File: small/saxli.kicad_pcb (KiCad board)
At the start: 4 copper layers, 160.5 x 102.4 mm, 191 parts, among them IC1 PIC32MX350F256H-V_PT, IC2 SIM808, J1 78800-0001, J10 Conn_01x06_Female, J11 Conn_Coaxial, J12 Conn_Coaxial, J2 Screw_Terminal_01x02, J3 Micro_SD_Card, J4 Conn_01x05_Female, J5 Conn_02x04_Odd_Even, J6 RJ45_Amphenol_RJMG1BD3B8K1ANR, J7 Screw_Terminal_01x08, J8 Screw_Terminal_01x08, J9 Screw_Terminal_01x08, Q1 2N7002, Q2 2N7002, Q3 2N7002, U1 LM358, U10 TPS5430DDAR, U11 EL357N(C)(TA)-G, U12 EL357N(C)(TA)-G, U13 ASSR-1218, U14 ST485EBDR, U15 ASSR-1218, U16 SRV05-4, U18 ULN2003A, U2 LM7805_TO220, U20 TPS5430DDAR, U3 LD1117S33TR_SOT223, U4 ENC28J60x-SS, U5 AT25M02, U6 EL357N(C)(TA)-G, U7 EL357N(C)(TA)-G, U8 PCF8563T, U9 ISO1540, Y1 Crystal, Y2 Crystal

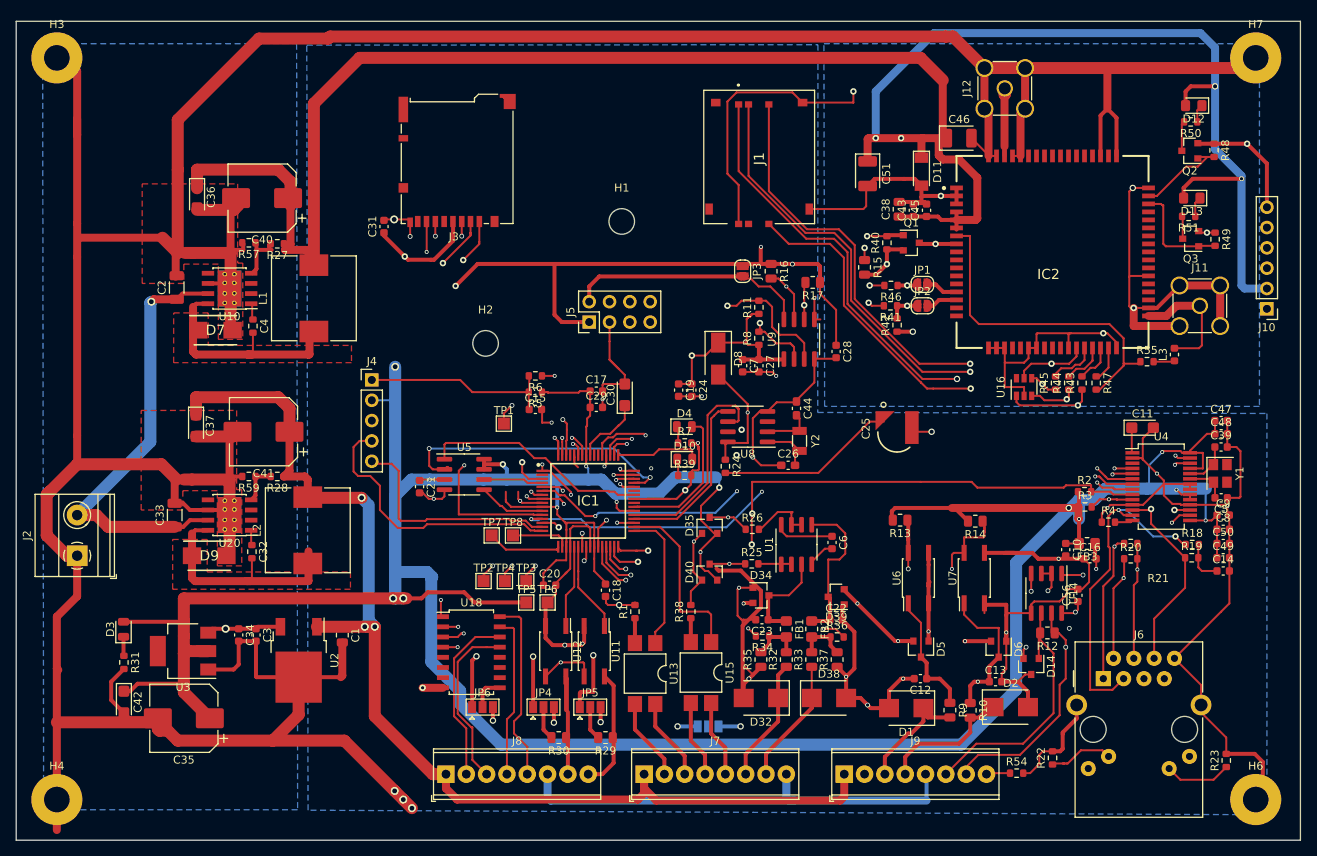
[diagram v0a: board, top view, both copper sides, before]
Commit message: ENC28j60 routed
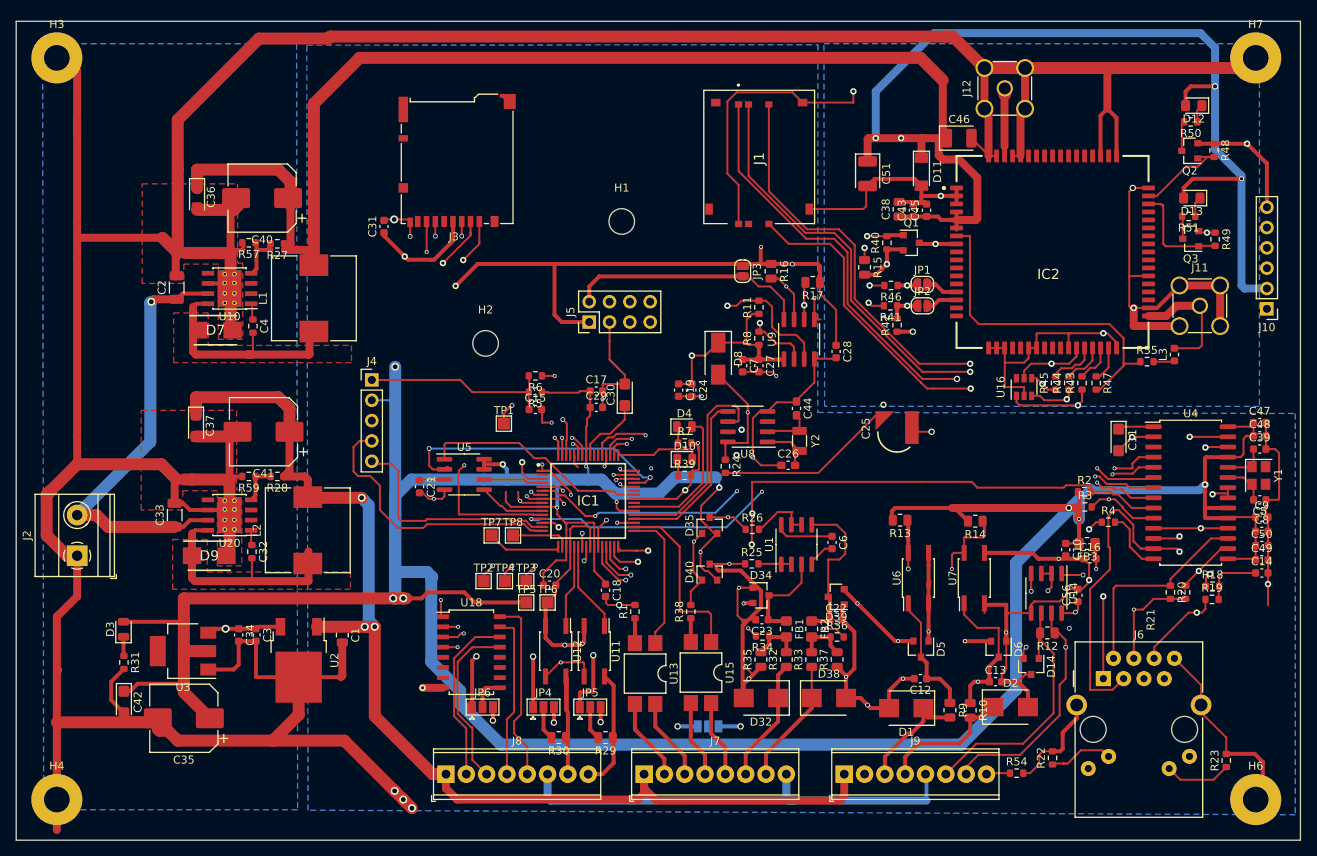
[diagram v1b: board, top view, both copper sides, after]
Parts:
- U4: footprint Package_SO:SSOP-28_5.3x10.2mm_P0.65mm -> Package_SO:SOIC-28W_7.5x17.9mm_P1.27mm
- moved R21 9.18 mm to (184.3, 92.2), turned to 270 degrees
- moved R20 6.49 mm to (182.4, 92.2), turned to 270 degrees
- moved R19 5.79 mm to (187.6, 93.1)
- moved R18 5.79 mm to (187.6, 91.4)
- moved C14 4.83 mm to (193.8, 89.8)
- moved C39 4.83 mm to (193.5, 74.3)
- moved C48 4.83 mm to (193.5, 72.6)
- moved C49 4.83 mm to (193.8, 88.1)
- moved C50 4.83 mm to (193.8, 86.4)
- moved C9 4.83 mm to (193.8, 82.8)
- moved C47 4.83 mm to (193.5, 71.0)
- moved C5 4.83 mm to (193.5, 80.6)
- moved C8 4.83 mm to (193.8, 84.6)
- moved Y1 4.83 mm to (193.4, 77.6)
- moved U4 3.76 mm to (184.9, 79.8)
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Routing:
- net GND: track 1186.3 -> 1162.0 mm, vias 43 -> 46
- net /etherne/LEDA: track 51.7 -> 59.7 mm
- net VDD3: track 548.7 -> 555.9 mm, vias 17 -> 15
- net /etherne/TPIN+: track 41.3 -> 47.5 mm
- net Net-(R4-Pad2): track 2.27 -> 7.97 mm
- net ENC_RST: track 82.3 -> 86.0 mm
- net ENC_INT: track 70.0 -> 73.6 mm
- net ENC_SS: track 84.5 -> 87.9 mm
- net SCK1: track 69.0 -> 72.1 mm
- net SDI1: track 123.9 -> 126.9 mm
- net ENC_WOL: track 68.3 -> 71.2 mm
- net Net-(C14-Pad1): track 5.40 -> 8.30 mm
- net SDO1: track 115.7 -> 118.5 mm
- net /etherne/TPOUT-: track 29.6 -> 31.2 mm
- net /etherne/LEDB: track 44.8 -> 46.3 mm
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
